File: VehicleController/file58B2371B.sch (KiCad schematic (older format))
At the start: 8 parts, among them Q3 Q_NMOS_GDS, U12 FGMMOPA6H, U13 U.FL_Antenna

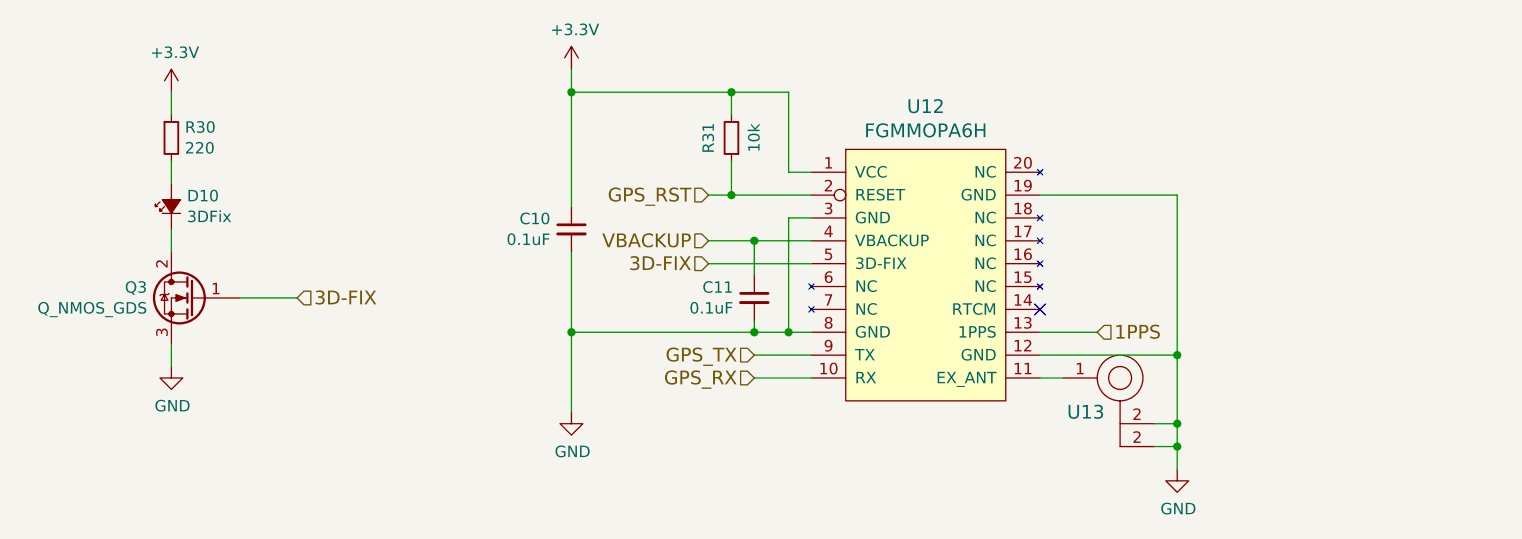
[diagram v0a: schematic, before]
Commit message: MX120, GDS->GSD FETs on VCU
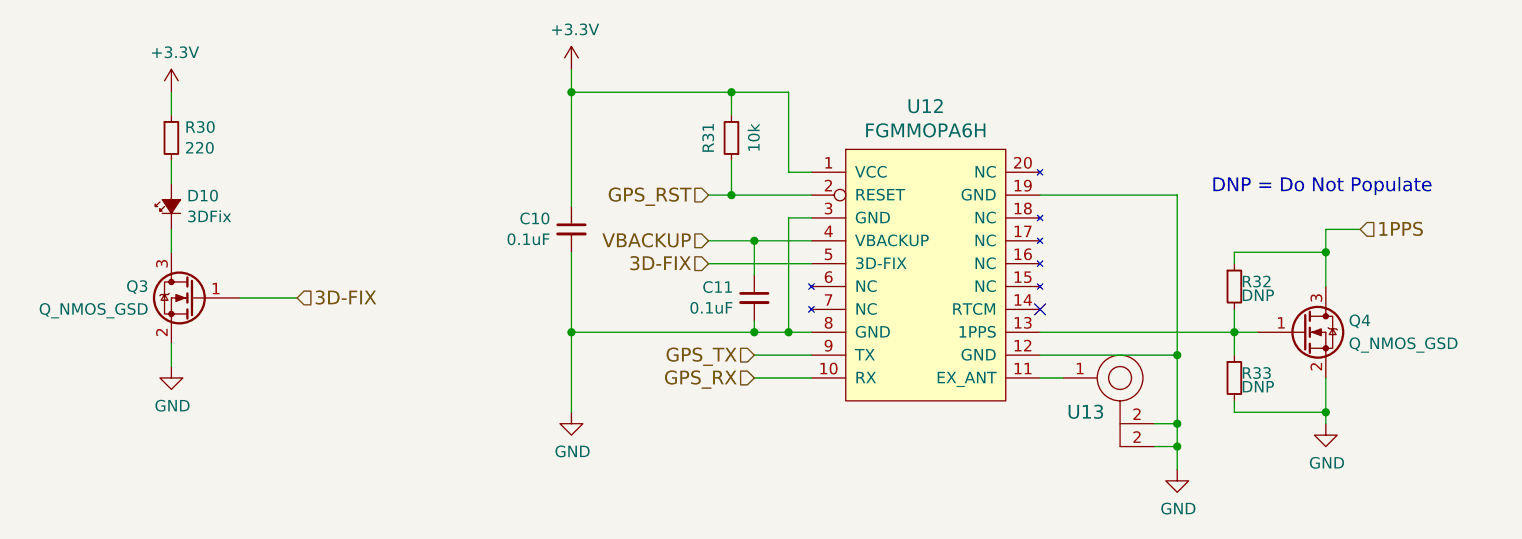
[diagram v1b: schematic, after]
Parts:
- removed Q3: Q_NMOS_GDS, TO_SOT_Packages_SMD:SOT-23_Handsoldering, symbol Q_NMOS_GDS
- added Q3, Q4: Q_NMOS_GSD, TO_SOT_Packages_SMD:SOT-23_Handsoldering, symbol Q_NMOS_GSD
- added R32, R33: DNP, Resistors_SMD:R_0805_HandSoldering, symbol R_Small
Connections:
- net 1PPS: now also Q4.3 (D), R32.1; no longer U12.13 (1PPS)
- net 3D-FIX: now also Q3.1 (G)
- net GND: now also Q3.2 (S), Q4.2 (S), R33.2
- net at D10.1 (K): now also Q3.3 (D)
- new net: Q4.1 (G), R32.2, R33.1, U12.13 (1PPS)
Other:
- note added: "DNP = Do Not Populate"
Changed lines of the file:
@@
 $EndComp
 $Comp
-L GND #PWR53
+L GND #PWR053
 U 1 1 58B24137
 P 5450 3800
-F 0 "#PWR53" H 5450 3550 50  0001 C CNN
+F 0 "#PWR053" H 5450 3550 50  0001 C CNN
 F 1 "GND" H 5455 3627 50  0000 C CNN
 F 2 "" H 5450 3800 50  0000 C CNN
@@
 $EndComp
 $Comp
-L GND #PWR54
+L GND #PWR054
 U 1 1 58B24148
 P 8100 4050
-F 0 "#PWR54" H 8100 3800 50  0001 C CNN
+F 0 "#PWR054" H 8100 3800 50  0001 C CNN
 F 1 "GND" H 8105 3877 50  0000 C CNN
 F 2 "" H 8100 4050 50  0000 C CNN
@@
 VBACKUP
 $Comp
-L +3.3V #PWR52
+L +3.3V #PWR055
 U 1 1 58B276E4
 P 5450 2300
-F 0 "#PWR52" H 5450 2150 50  0001 C CNN
+F 0 "#PWR055" H 5450 2150 50  0001 C CNN
 F 1 "+3.3V" H 5465 2473 50  0000 C CNN
 F 2 "" H 5450 2300 50  0000 C CNN
@@
 $EndComp
 $Comp
-L GND #PWR51
+L GND #PWR056
 U 1 1 58B23C84
 P 3700 3600
-F 0 "#PWR51" H 3700 3350 50  0001 C CNN
+F 0 "#PWR056" H 3700 3350 50  0001 C CNN
 F 1 "GND" H 3705 3427 50  0000 C CNN
 F 2 "" H 3700 3600 50  0000 C CNN
@@
 $EndComp
 $Comp
-L Q_NMOS_GDS Q3
-U 1 1 58B23C7C
-P 3800 3300
-F 0 "Q3" H 4006 3346 50  0000 L CNN
-F 1 "Q_NMOS_GDS" H 4006 3255 50  0000 L CNN
-F 2 "TO_SOT_Packages_SMD:SOT-23_Handsoldering" H 4000 3400 50  0001 C CNN
-F 3 "" H 3800 3300 50  0000 C CNN
-	1    3800 3300
-	-1   0    0    -1
-$EndComp
-$Comp
-L +3.3V #PWR50
+L +3.3V #PWR057
 U 1 1 58B23C75
 P 3700 2400
-F 0 "#PWR50" H 3700 2250 50  0001 C CNN
+F 0 "#PWR057" H 3700 2250 50  0001 C CNN
 F 1 "+3.3V" H 3715 2573 50  0000 C CNN
 F 2 "" H 3700 2400 50  0000 C CNN
@@
 Text HLabel 4250 3300 2    60   Input ~ 0
 3D-FIX
-Text HLabel 7750 3450 2    60   Input ~ 0
+Text HLabel 8900 3000 2    60   Input ~ 0
 1PPS
 Text HLabel 6050 2850 0    60   Input ~ 0
@@
 Connection ~ 8100 3850
 Wire Wire Line
-	7500 3450 7750 3450
+	7500 3450 8450 3450
 Wire Wire Line
 	7500 3550 8100 3550
@@
 	0    -1   -1   0
 $EndComp
+$Comp
+L Q_NMOS_GSD Q3
+U 1 1 591E7689
+P 3800 3300
+F 0 "Q3" H 4000 3350 50  0000 L CNN
+F 1 "Q_NMOS_GSD" H 4000 3250 50  0000 L CNN
+F 2 "TO_SOT_Packages_SMD:SOT-23_Handsoldering" H 4000 3400 50  0001 C CNN
+F 3 "" H 3800 3300 50  0001 C CNN
+	1    3800 3300
+	-1   0    0    -1
+$EndComp
+$Comp
+L Q_NMOS_GSD Q4
+U 1 1 59218AFB
+P 8650 3450
+F 0 "Q4" H 8850 3500 50  0000 L CNN
+F 1 "Q_NMOS_GSD" H 8850 3400 50  0000 L CNN
+F 2 "TO_SOT_Packages_SMD:SOT-23_Handsoldering" H 8850 3550 50  0001 C CNN
+F 3 "" H 8650 3450 50  0001 C CNN
+	1    8650 3450
+	1    0    0    -1
+$EndComp
+Wire Wire Line
+	8900 3000 8750 3000
+Wire Wire Line
+	8750 3000 8750 3250
+$Comp
+L GND #PWR058
+U 1 1 59218D57
+P 8750 3850
+F 0 "#PWR058" H 8750 3600 50  0001 C CNN
+F 1 "GND" H 8755 3677 50  0000 C CNN
+F 2 "" H 8750 3850 50  0000 C CNN
+F 3 "" H 8750 3850 50  0000 C CNN
+	1    8750 3850
+	1    0    0    -1
+$EndComp
+Wire Wire Line
+	8750 3850 8750 3650
+$Comp
+L R_Small R32
+U 1 1 59219167
+P 8350 3250
+F 0 "R32" H 8380 3270 50  0000 L CNN
+F 1 "DNP" H 8380 3210 50  0000 L CNN
+F 2 "Resistors_SMD:R_0805_HandSoldering" H 8350 3250 50  0001 C CNN
+F 3 "" H 8350 3250 50  0001 C CNN
+	1    8350 3250
+	1    0    0    -1
+$EndComp
+Wire Wire Line
+	8350 3150 8350 3100
+Wire Wire Line
+	8350 3100 8750 3100
+Connection ~ 8750 3100
+Wire Wire Line
+	8350 3350 8350 3550
+Connection ~ 8350 3450
+$Comp
+L R_Small R33
+U 1 1 5921923E
+P 8350 3650
+F 0 "R33" H 8380 3670 50  0000 L CNN
+F 1 "DNP" H 8380 3610 50  0000 L CNN
+F 2 "Resistors_SMD:R_0805_HandSoldering" H 8350 3650 50  0001 C CNN
+F 3 "" H 8350 3650 50  0001 C CNN
+	1    8350 3650
+	1    0    0    -1
+$EndComp
+Wire Wire Line
+	8350 3750 8350 3800
+Wire Wire Line
+	8350 3800 8750 3800
+Connection ~ 8750 3800
+Text Notes 8250 2850 0    60   ~ 0
+DNP = Do Not Populate
 $EndSCHEMATC

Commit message: Revert "MX120, GDS->GSD FETs on VCU"
This reverts commit 5f93bf7ab8a0e63cb004bd031bee3d8b2541593f.
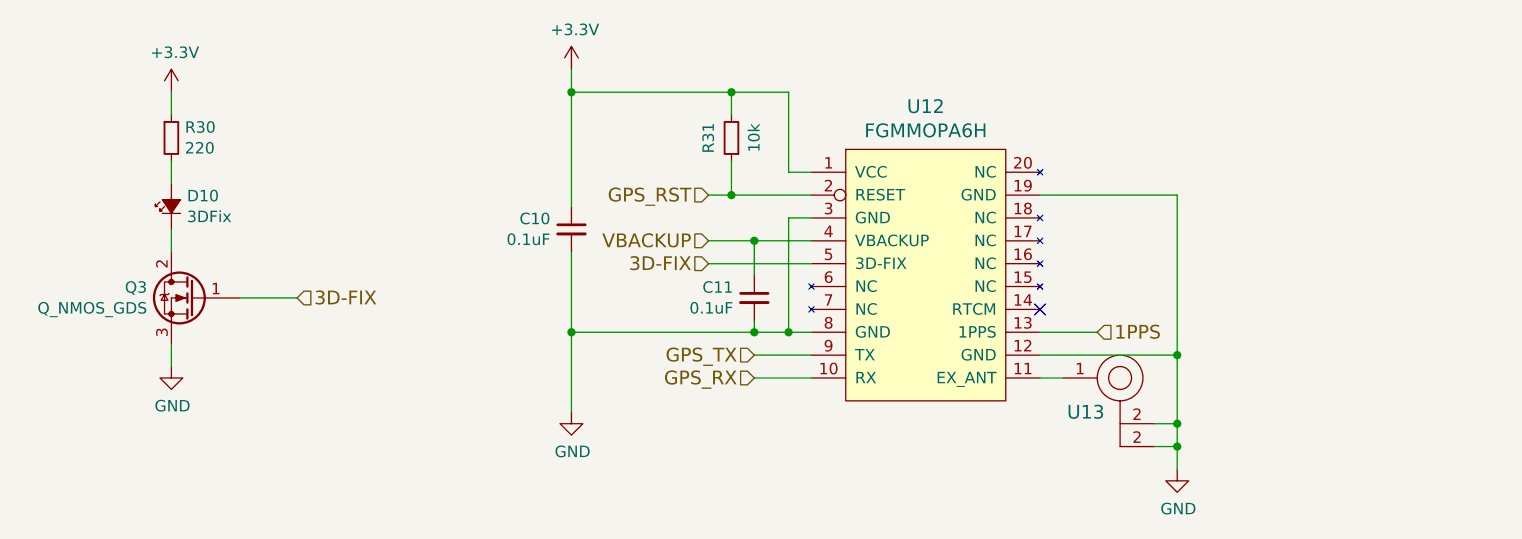
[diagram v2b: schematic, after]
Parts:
- removed Q3, Q4: Q_NMOS_GSD, TO_SOT_Packages_SMD:SOT-23_Handsoldering, symbol Q_NMOS_GSD
- removed R32, R33: DNP, Resistors_SMD:R_0805_HandSoldering, symbol R_Small
- added Q3: Q_NMOS_GDS, TO_SOT_Packages_SMD:SOT-23_Handsoldering, symbol Q_NMOS_GDS
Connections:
- net 1PPS: now also U12.13 (1PPS)
- net 3D-FIX: now also Q3.1 (G)
- net GND: now also Q3.3 (S)
- net at D10.1 (K): now also Q3.2 (D)
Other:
- note removed: "DNP = Do Not Populate"
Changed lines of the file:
@@
 $EndComp
 $Comp
-L GND #PWR053
+L GND #PWR53
 U 1 1 58B24137
 P 5450 3800
-F 0 "#PWR053" H 5450 3550 50  0001 C CNN
+F 0 "#PWR53" H 5450 3550 50  0001 C CNN
 F 1 "GND" H 5455 3627 50  0000 C CNN
 F 2 "" H 5450 3800 50  0000 C CNN
@@
 $EndComp
 $Comp
-L GND #PWR054
+L GND #PWR54
 U 1 1 58B24148
 P 8100 4050
-F 0 "#PWR054" H 8100 3800 50  0001 C CNN
+F 0 "#PWR54" H 8100 3800 50  0001 C CNN
 F 1 "GND" H 8105 3877 50  0000 C CNN
 F 2 "" H 8100 4050 50  0000 C CNN
@@
 VBACKUP
 $Comp
-L +3.3V #PWR055
+L +3.3V #PWR52
 U 1 1 58B276E4
 P 5450 2300
-F 0 "#PWR055" H 5450 2150 50  0001 C CNN
+F 0 "#PWR52" H 5450 2150 50  0001 C CNN
 F 1 "+3.3V" H 5465 2473 50  0000 C CNN
 F 2 "" H 5450 2300 50  0000 C CNN
@@
 $EndComp
 $Comp
-L GND #PWR056
+L GND #PWR51
 U 1 1 58B23C84
 P 3700 3600
-F 0 "#PWR056" H 3700 3350 50  0001 C CNN
+F 0 "#PWR51" H 3700 3350 50  0001 C CNN
 F 1 "GND" H 3705 3427 50  0000 C CNN
 F 2 "" H 3700 3600 50  0000 C CNN
@@
 $EndComp
 $Comp
-L +3.3V #PWR057
+L Q_NMOS_GDS Q3
+U 1 1 58B23C7C
+P 3800 3300
+F 0 "Q3" H 4006 3346 50  0000 L CNN
+F 1 "Q_NMOS_GDS" H 4006 3255 50  0000 L CNN
+F 2 "TO_SOT_Packages_SMD:SOT-23_Handsoldering" H 4000 3400 50  0001 C CNN
+F 3 "" H 3800 3300 50  0000 C CNN
+	1    3800 3300
+	-1   0    0    -1
+$EndComp
+$Comp
+L +3.3V #PWR50
 U 1 1 58B23C75
 P 3700 2400
-F 0 "#PWR057" H 3700 2250 50  0001 C CNN
+F 0 "#PWR50" H 3700 2250 50  0001 C CNN
 F 1 "+3.3V" H 3715 2573 50  0000 C CNN
 F 2 "" H 3700 2400 50  0000 C CNN
@@
 Text HLabel 4250 3300 2    60   Input ~ 0
 3D-FIX
-Text HLabel 8900 3000 2    60   Input ~ 0
+Text HLabel 7750 3450 2    60   Input ~ 0
 1PPS
 Text HLabel 6050 2850 0    60   Input ~ 0
@@
 Connection ~ 8100 3850
 Wire Wire Line
-	7500 3450 8450 3450
+	7500 3450 7750 3450
 Wire Wire Line
 	7500 3550 8100 3550
@@
 	0    -1   -1   0
 $EndComp
-$Comp
-L Q_NMOS_GSD Q3
-U 1 1 591E7689
-P 3800 3300
-F 0 "Q3" H 4000 3350 50  0000 L CNN
-F 1 "Q_NMOS_GSD" H 4000 3250 50  0000 L CNN
-F 2 "TO_SOT_Packages_SMD:SOT-23_Handsoldering" H 4000 3400 50  0001 C CNN
-F 3 "" H 3800 3300 50  0001 C CNN
-	1    3800 3300
-	-1   0    0    -1
-$EndComp
-$Comp
-L Q_NMOS_GSD Q4
-U 1 1 59218AFB
-P 8650 3450
-F 0 "Q4" H 8850 3500 50  0000 L CNN
-F 1 "Q_NMOS_GSD" H 8850 3400 50  0000 L CNN
-F 2 "TO_SOT_Packages_SMD:SOT-23_Handsoldering" H 8850 3550 50  0001 C CNN
-F 3 "" H 8650 3450 50  0001 C CNN
-	1    8650 3450
-	1    0    0    -1
-$EndComp
-Wire Wire Line
-	8900 3000 8750 3000
-Wire Wire Line
-	8750 3000 8750 3250
-$Comp
-L GND #PWR058
-U 1 1 59218D57
-P 8750 3850
-F 0 "#PWR058" H 8750 3600 50  0001 C CNN
-F 1 "GND" H 8755 3677 50  0000 C CNN
-F 2 "" H 8750 3850 50  0000 C CNN
-F 3 "" H 8750 3850 50  0000 C CNN
-	1    8750 3850
-	1    0    0    -1
-$EndComp
-Wire Wire Line
-	8750 3850 8750 3650
-$Comp
-L R_Small R32
-U 1 1 59219167
-P 8350 3250
-F 0 "R32" H 8380 3270 50  0000 L CNN
-F 1 "DNP" H 8380 3210 50  0000 L CNN
-F 2 "Resistors_SMD:R_0805_HandSoldering" H 8350 3250 50  0001 C CNN
-F 3 "" H 8350 3250 50  0001 C CNN
-	1    8350 3250
-	1    0    0    -1
-$EndComp
-Wire Wire Line
-	8350 3150 8350 3100
-Wire Wire Line
-	8350 3100 8750 3100
-Connection ~ 8750 3100
-Wire Wire Line
-	8350 3350 8350 3550
-Connection ~ 8350 3450
-$Comp
-L R_Small R33
-U 1 1 5921923E
-P 8350 3650
-F 0 "R33" H 8380 3670 50  0000 L CNN
-F 1 "DNP" H 8380 3610 50  0000 L CNN
-F 2 "Resistors_SMD:R_0805_HandSoldering" H 8350 3650 50  0001 C CNN
-F 3 "" H 8350 3650 50  0001 C CNN
-	1    8350 3650
-	1    0    0    -1
-$EndComp
-Wire Wire Line
-	8350 3750 8350 3800
-Wire Wire Line
-	8350 3800 8750 3800
-Connection ~ 8750 3800
-Text Notes 8250 2850 0    60   ~ 0
-DNP = Do Not Populate
 $EndSCHEMATC
